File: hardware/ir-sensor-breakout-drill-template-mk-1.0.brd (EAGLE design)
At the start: 24 x 29 mm, 6 parts, among them U1 MLX906145V-PTH

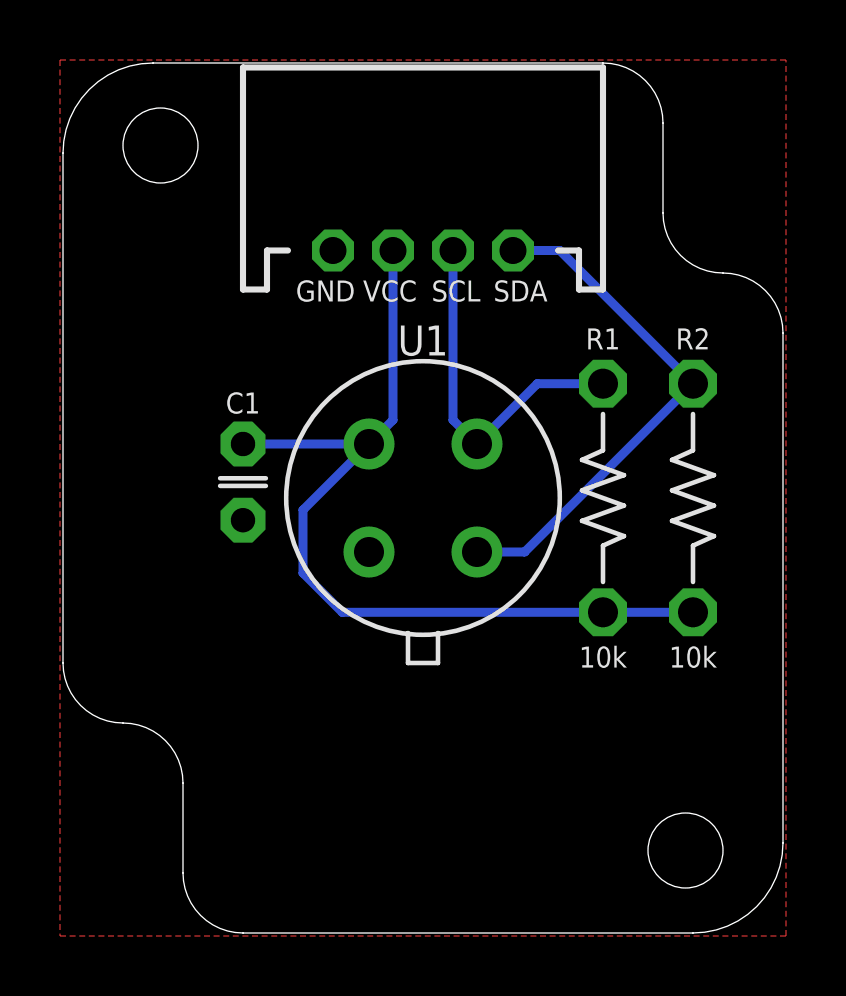
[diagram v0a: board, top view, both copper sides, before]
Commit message: twiddling around with IR sensor breakouts
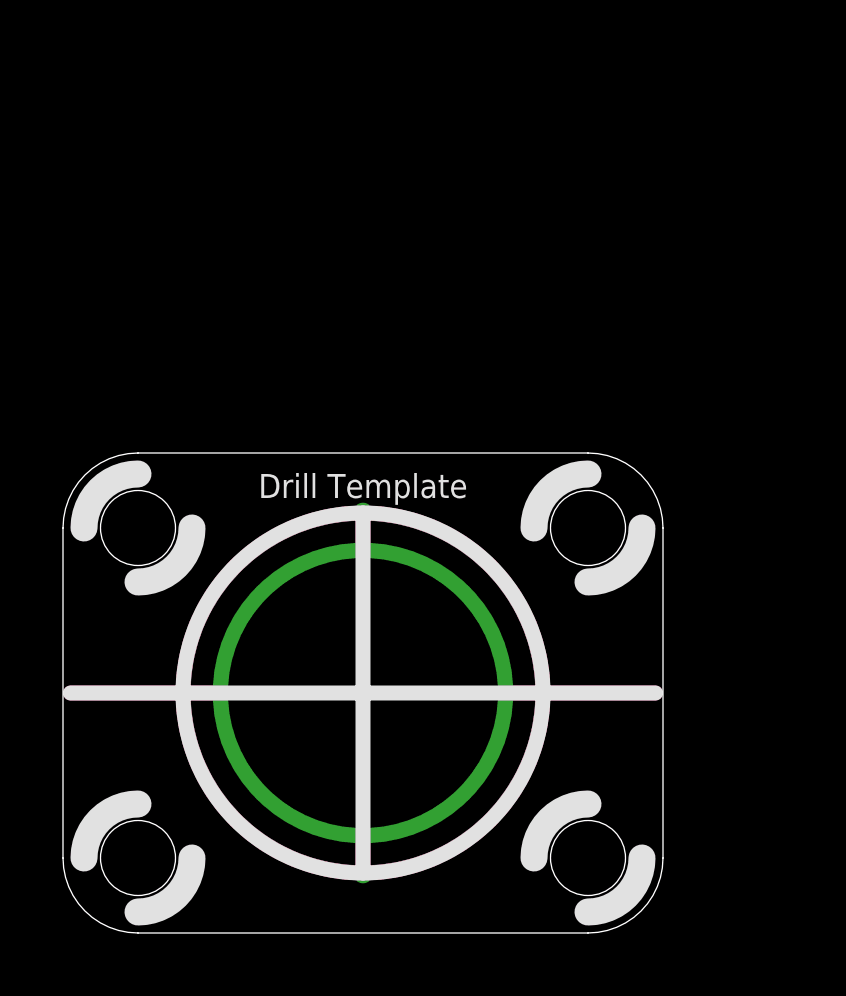
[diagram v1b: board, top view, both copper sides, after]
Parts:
- removed C1: 0.1uF, A_butts:C025-024X044
- removed JP1: M04JST-PTH, A_butts:JST-4-PH-RA-PTH
- removed R1, R2: 10k, A_butts:RESISTOR-AXIAL-PTH-7.62MM
- removed U1: MLX906145V-PTH, A_butts:TO-39-4
- added H1, H2, H3, H4: HOLE#2, A_butts:HOLE-#2
- FRAME1: value (none) -> FRAME-LETTERNO_PACKAGE
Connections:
- removed net GND: C1.2, JP1.1, U1.4
- removed net SCL: JP1.4, R2.P$1, U1.1
- removed net SDA: JP1.3, R1.P$1, U1.2
- removed net VCC: C1.1, JP1.2, R1.P$2, R2.P$2, U1.3
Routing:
- net GND: track 0.00 -> 130.9 mm, vias 0 -> 5
- net VCC: track 29.7 -> 0.00 mm
- net SCL: track 17.4 -> 0.00 mm
- net SDA: track 11.8 -> 0.00 mm
- removed copper zone on layer 1, net GND
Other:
- board size 24 x 29 mm -> 20 x 16 mm
- board text added: ">VERSION"
- board text added: "Drill Template"
- board text removed: "GND"
- board text removed: "SCL"
- board text removed: "SDA"
- board text removed: "VCC"
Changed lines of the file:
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@@
 <setting verticaltext="up"/>
 </settings>
-<grid distance="0.5" unitdist="mm" unit="mm" style="lines" multiple="2" display="yes" altdistance="1" altunitdist="mil" altunit="mil"/>
+<grid distance="0.25" unitdist="mm" unit="mm" style="lines" multiple="4" display="yes" altdistance="1" altunitdist="mil" altunit="mil"/>
 <layers>
 <layer number="1" name="Top" color="4" fill="1" visible="yes" active="yes"/>
@@
 <board>
 <plain>
-<wire x1="0" y1="26" x2="0" y2="9" width="0" layer="20"/>
-<wire x1="0" y1="9" x2="2" y2="7" width="0" layer="20" curve="90"/>
-<wire x1="2" y1="7" x2="4" y2="5" width="0" layer="20" curve="-90"/>
-<wire x1="4" y1="5" x2="4" y2="2" width="0" layer="20"/>
-<wire x1="4" y1="2" x2="6" y2="0" width="0" layer="20" curve="90"/>
-<wire x1="6" y1="0" x2="21" y2="0" width="0" layer="20"/>
-<wire x1="21" y1="0" x2="24" y2="3" width="0" layer="20" curve="90"/>
-<wire x1="22" y1="22" x2="24" y2="20" width="0" layer="20" curve="-90"/>
-<wire x1="24" y1="20" x2="24" y2="3" width="0" layer="20"/>
-<wire x1="20" y1="27" x2="20" y2="24" width="0" layer="20"/>
-<wire x1="20" y1="24" x2="22" y2="22" width="0" layer="20" curve="90"/>
-<wire x1="20" y1="27" x2="18" y2="29" width="0" layer="20" curve="90"/>
-<wire x1="18" y1="29" x2="3" y2="29" width="0" layer="20"/>
-<wire x1="3" y1="29" x2="0" y2="26" width="0" layer="20" curve="90"/>
-<hole x="20.75" y="2.75" drill="2.5"/>
-<hole x="3.25" y="26.25" drill="2.5"/>
-<text x="8.75" y="21.75" size="0.7" layer="21" font="vector" ratio="12" align="top-center">GND</text>
-<text x="10.9" y="21.75" size="0.7" layer="21" font="vector" ratio="12" align="top-center">VCC</text>
-<text x="15.25" y="21.75" size="0.7" layer="21" font="vector" ratio="12" align="top-center">SDA</text>
-<text x="13.1" y="21.75" size="0.7" layer="21" font="vector" ratio="12" align="top-center">SCL</text>
-<text x="8.75" y="21.75" size="0.7" layer="22" font="vector" ratio="12" rot="MR180" align="bottom-center">GND</text>
-<text x="10.9" y="21.75" size="0.7" layer="22" font="vector" ratio="12" rot="MR180" align="bottom-center">VCC</text>
-<text x="15.25" y="21.75" size="0.7" layer="22" font="vector" ratio="12" rot="MR180" align="bottom-center">SDA</text>
-<text x="13.1" y="21.75" size="0.7" layer="22" font="vector" ratio="12" rot="MR180" align="bottom-center">SCL</text>
+<wire x1="2.5" y1="16" x2="17.5" y2="16" width="0" layer="20"/>
+<wire x1="17.5" y1="16" x2="20" y2="13.5" width="0" layer="20" curve="-90"/>
+<wire x1="2.5" y1="0" x2="17.5" y2="0" width="0" layer="20"/>
+<wire x1="17.5" y1="0" x2="20" y2="2.5" width="0" layer="20" curve="90"/>
+<wire x1="20" y1="2.5" x2="20" y2="13.5" width="0" layer="20"/>
+<wire x1="2.5" y1="16" x2="0" y2="13.5" width="0" layer="20" curve="90"/>
+<wire x1="0" y1="13.5" x2="0" y2="2.5" width="0" layer="20"/>
+<wire x1="0" y1="2.5" x2="2.5" y2="0" width="0" layer="20" curve="90"/>
+<text x="6" y="1" size="0.6" layer="22" font="vector" ratio="12" rot="MR180" align="top-center">&gt;VERSION</text>
+<text x="14" y="1" size="0.6" layer="21" font="vector" ratio="12" rot="R180" align="top-center">&gt;VERSION</text>
+<wire x1="0.25" y1="8" x2="19.75" y2="8" width="0.5" layer="21"/>
+<wire x1="10" y1="14" x2="10" y2="2" width="0.5" layer="21"/>
+<wire x1="0.25" y1="8" x2="19.75" y2="8" width="0.5" layer="22"/>
+<wire x1="10" y1="14" x2="10" y2="2" width="0.5" layer="22"/>
+<circle x="10" y="8" radius="6" width="0.5" layer="21"/>
+<circle x="10" y="8" radius="6" width="0.5" layer="22"/>
+<text x="10" y="14.5" size="0.8" layer="21" font="vector" ratio="12" align="bottom-center">Drill Template</text>
+<text x="10" y="14.5" size="0.8" layer="22" font="vector" ratio="12" rot="MR0" align="bottom-center">Drill Template</text>
 </plain>
 <attributes>
+<attribute name="VERSION" value="v1.0"/>
 </attributes>
 <variantdefs>
@@
 </autorouter>
 <elements>
-<element name="FRAME1" library="A_butts" package="DUMMY" value="" x="0" y="0">
+<element name="FRAME1" library="A_butts" package="DUMMY" value="FRAME-LETTERNO_PACKAGE" x="0" y="0">
 <attribute name="VERSION" value="v01" x="0" y="0" size="0.5" layer="27" font="vector" ratio="12" display="off"/>
 <attribute name="DESIGNER" value="Nobody" x="0" y="0" size="0.5" layer="27" font="vector" ratio="12" display="off"/>
 </element>
-<element name="JP1" library="A_butts" package="JST-4-PH-RA-PTH" value="M04JST-PTH" x="9" y="22.75" smashed="yes">
-<attribute name="SKU" value="PRT-09916" x="9" y="22.75" size="1.778" layer="27" display="off"/>
-</element>
-<element name="U1" library="A_butts" package="TO-39-4" value="MLX906145V-PTH" x="12" y="14.5" smashed="yes" rot="R180">
-<attribute name="NAME" x="12" y="19.25" size="1" layer="25" font="vector" ratio="12" rot="R180" align="top-center"/>
-</element>
-<element name="C1" library="A_butts" package="C025-024X044" value="0.1uF" x="6" y="15.03" rot="R270"/>
-<element name="R1" library="A_butts" package="RESISTOR-AXIAL-PTH-7.62MM" value="10k" x="18" y="14.5" rot="R270"/>
-<element name="R2" library="A_butts" package="RESISTOR-AXIAL-PTH-7.62MM" value="10k" x="21" y="14.5" rot="R270"/>
+<element name="H1" library="A_butts" package="HOLE-#2" value="HOLE#2" x="2.5" y="2.5"/>
+<element name="H2" library="A_butts" package="HOLE-#2" value="HOLE#2" x="2.5" y="13.5"/>
+<element name="H3" library="A_butts" package="HOLE-#2" value="HOLE#2" x="17.5" y="13.5"/>
+<element name="H4" library="A_butts" package="HOLE-#2" value="HOLE#2" x="17.5" y="2.5"/>
 </elements>
 <signals>
-<signal name="VCC">
-<contactref element="C1" pad="1"/>
-<contactref element="R1" pad="P$2"/>
-<contactref element="R2" pad="P$2"/>
-<contactref element="JP1" pad="2"/>
-<contactref element="U1" pad="3"/>
-<wire x1="11" y1="22.75" x2="11" y2="17.1" width="0.3" layer="16"/>
-<wire x1="11" y1="17.1" x2="10.2" y2="16.3" width="0.3" layer="16"/>
-<wire x1="6" y1="16.3" x2="10.2" y2="16.3" width="0.3" layer="16"/>
-<wire x1="10.2" y1="16.3" x2="8" y2="14.1" width="0.3" layer="16"/>
-<wire x1="8" y1="14.1" x2="8" y2="12" width="0.3" layer="16"/>
-<wire x1="8" y1="12" x2="9.31" y2="10.69" width="0.3" layer="16"/>
-<wire x1="9.31" y1="10.69" x2="18" y2="10.69" width="0.3" layer="16"/>
-<wire x1="18" y1="10.69" x2="21" y2="10.69" width="0.3" layer="16"/>
-</signal>
 <signal name="GND">
-<contactref element="C1" pad="2"/>
-<contactref element="JP1" pad="1"/>
-<contactref element="U1" pad="4"/>
-<polygon width="0.1524" layer="1">
-<vertex x="-0.1" y="-0.1"/>
-<vertex x="24.1" y="-0.1"/>
-<vertex x="24.1" y="29.1"/>
-<vertex x="-0.1" y="29.1"/>
-</polygon>
-</signal>
-<signal name="SDA">
-<contactref element="JP1" pad="3"/>
-<contactref element="U1" pad="2"/>
-<contactref element="R1" pad="P$1"/>
-<wire x1="13" y1="22.75" x2="13" y2="17.1" width="0.3" layer="16"/>
-<wire x1="13" y1="17.1" x2="13.8" y2="16.3" width="0.3" layer="16"/>
-<wire x1="13.8" y1="16.3" x2="15.81" y2="18.31" width="0.3" layer="16"/>
-<wire x1="15.81" y1="18.31" x2="18" y2="18.31" width="0.3" layer="16"/>
-</signal>
-<signal name="SCL">
-<contactref element="JP1" pad="4"/>
-<contactref element="U1" pad="1"/>
-<contactref element="R2" pad="P$1"/>
-<wire x1="15" y1="22.75" x2="16.56" y2="22.75" width="0.3" layer="16"/>
-<wire x1="16.56" y1="22.75" x2="21" y2="18.31" width="0.3" layer="16"/>
-<wire x1="13.8" y1="12.7" x2="15.39" y2="12.7" width="0.3" layer="16"/>
-<wire x1="15.39" y1="12.7" x2="21" y2="18.31" width="0.3" layer="16"/>
+<via x="10" y="8" extent="1-16" drill="9"/>
+<wire x1="0.25" y1="8" x2="4" y2="8" width="0.5" layer="16"/>
+<wire x1="4" y1="8" x2="16" y2="8" width="0.5" layer="16"/>
+<wire x1="16" y1="8" x2="19.75" y2="8" width="0.5" layer="16"/>
+<wire x1="10" y1="2" x2="10" y2="14" width="0.5" layer="16"/>
+<wire x1="10" y1="8" x2="10" y2="2" width="0.5" layer="1"/>
+<wire x1="0.25" y1="8" x2="4" y2="8" width="0.5" layer="1"/>
+<wire x1="4" y1="8" x2="10" y2="8" width="0.5" layer="1"/>
+<wire x1="16" y1="8" x2="19.75" y2="8" width="0.5" layer="1"/>
+<via x="4" y="8" extent="1-16" drill="0.3302"/>
+<via x="10" y="14" extent="1-16" drill="0.3302"/>
+<via x="16" y="8" extent="1-16" drill="0.3302"/>
+<via x="10" y="2" extent="1-16" drill="0.3302"/>
+<wire x1="10" y1="8" x2="10" y2="14" width="0.5" layer="1"/>
+<wire x1="10" y1="8" x2="16" y2="8" width="0.5" layer="1"/>
+<wire x1="4" y1="8" x2="10" y2="14" width="0.5" layer="1" curve="-90"/>
+<wire x1="10" y1="14" x2="16" y2="8" width="0.5" layer="1" curve="-90"/>
+<wire x1="16" y1="8" x2="10" y2="2" width="0.5" layer="1" curve="-90"/>
+<wire x1="10" y1="2" x2="4" y2="8" width="0.5" layer="1" curve="-90"/>
+<wire x1="4" y1="8" x2="10" y2="2" width="0.5" layer="16" curve="90"/>
+<wire x1="10" y1="2" x2="16" y2="8" width="0.5" layer="16" curve="90"/>
+<wire x1="16" y1="8" x2="10" y2="14" width="0.5" layer="16" curve="90"/>
+<wire x1="10" y1="14" x2="4" y2="8" width="0.5" layer="16" curve="90"/>
 </signal>
 </signals>
+<errors>
+</errors>
 </board>
 </drawing>
